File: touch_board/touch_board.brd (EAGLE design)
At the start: 81 x 62.2 mm, 51 parts, among them IC1 PIC18F47K42-I_PT, IC2 MAX203EEWP, K1 G6K-2P, X1 RS-232-1, X2 RS-232-2, X5 Relay conn, X6 MINI-USB-UX60A-MB-5ST

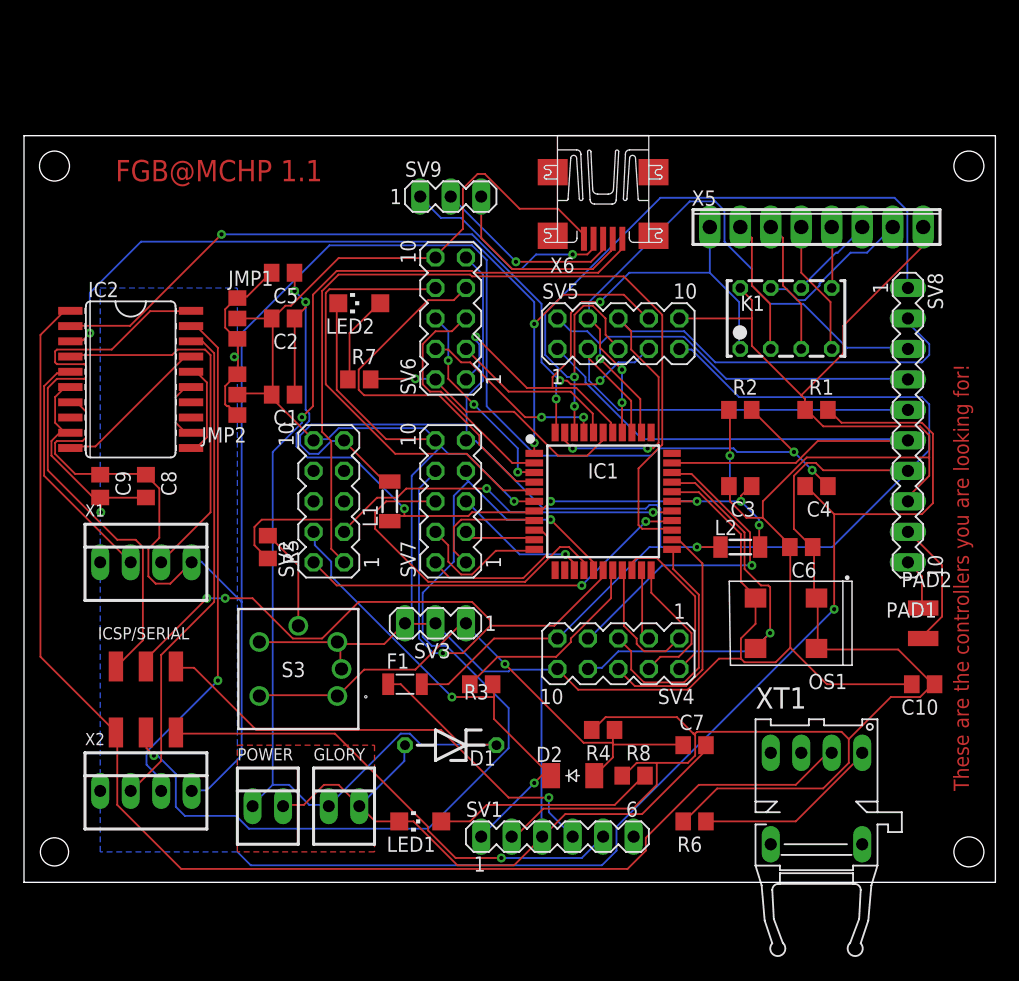
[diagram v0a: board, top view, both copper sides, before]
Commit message: update
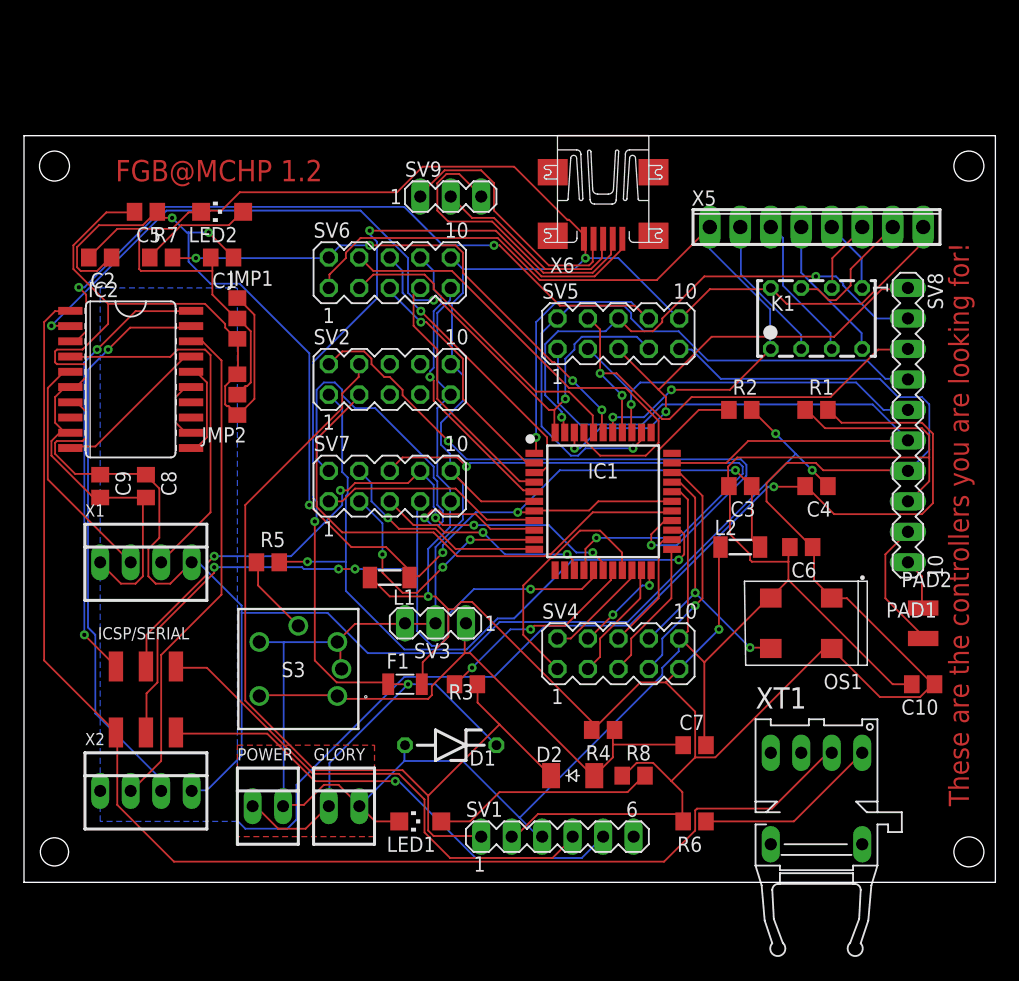
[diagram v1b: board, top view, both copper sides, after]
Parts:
- moved R7 19.4 mm to (26.7, 69.8)
- moved C2 16.1 mm to (21.6, 69.8)
- moved LED2 13.7 mm to (31.8, 73.7)
- moved C5 12.5 mm to (25.4, 73.7)
- moved C1 12.5 mm to (31.8, 69.8)
- moved SV2 11.4 mm to (45.7, 59.7), turned to 0 degrees
- moved L1 6.35 mm to (45.7, 43.2), turned to 180 degrees
- moved SV6 6.35 mm to (45.7, 68.6), turned to 0 degrees
- moved SV7 5.24 mm to (45.7, 50.8), turned to 0 degrees
- moved K1 2.54 mm to (80.0, 64.8)
- moved OS1 1.27 mm to (80.0, 39.4)
- moved R3 1.27 mm to (52.1, 34.3)
- moved R5 1.27 mm to (35.6, 44.5), turned to 0 degrees
- turned SV4 to 0 degrees
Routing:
- net VDD: track 252.6 -> 207.2 mm, vias 1 -> 2
- net GND: track 130.3 -> 173.8 mm, vias 3 -> 1
- net N$58: track 81.4 -> 123.8 mm, vias 8 -> 6
- net N$2: track 40.2 -> 76.7 mm, vias 2 -> 0
- net VCC: track 148.7 -> 116.7 mm
- net N$4: track 84.8 -> 59.0 mm, vias 0 -> 2
- net N$41: track 16.0 -> 40.2 mm, vias 2 -> 0
- net N$47: track 13.5 -> 37.3 mm, vias 0 -> 1
- net N$63: track 63.9 -> 41.4 mm
- net N$10: track 23.3 -> 44.8 mm, vias 1 -> 4
- net N$5: track 32.9 -> 54.1 mm
- net N$51: track 28.4 -> 48.6 mm, vias 0 -> 2
- net N$7: track 81.0 -> 63.3 mm, vias 2 -> 4
- net N$52: track 50.4 -> 66.7 mm
- net N$48: track 6.05 -> 22.0 mm, vias 0 -> 3
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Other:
- board text added: "FGB@MCHP 1.2"
- board text removed: "FGB@MCHP 1.1"
